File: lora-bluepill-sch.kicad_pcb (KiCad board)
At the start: 2 copper layers, 100 x 80 mm, 63 parts, among them J1 Conn_01x05, J10 Screw_Terminal_01x04, J11 Screw_Terminal_01x04, J2 Conn_01x05, J4 Conn_01x04_Male, J5 Conn_01x02, J7 Screw_Terminal_01x02, J8 Screw_Terminal_01x02, Q1 BC558, U10 YAAJ_WeAct_BlackPill_Part_Like, U2 FTDI_Breakout, U3 RadioEnge_LoRaWAN, U4 PC817, U5 PC817, U6 PC817, U7 PC817, U8 PC817, U9 NE555P

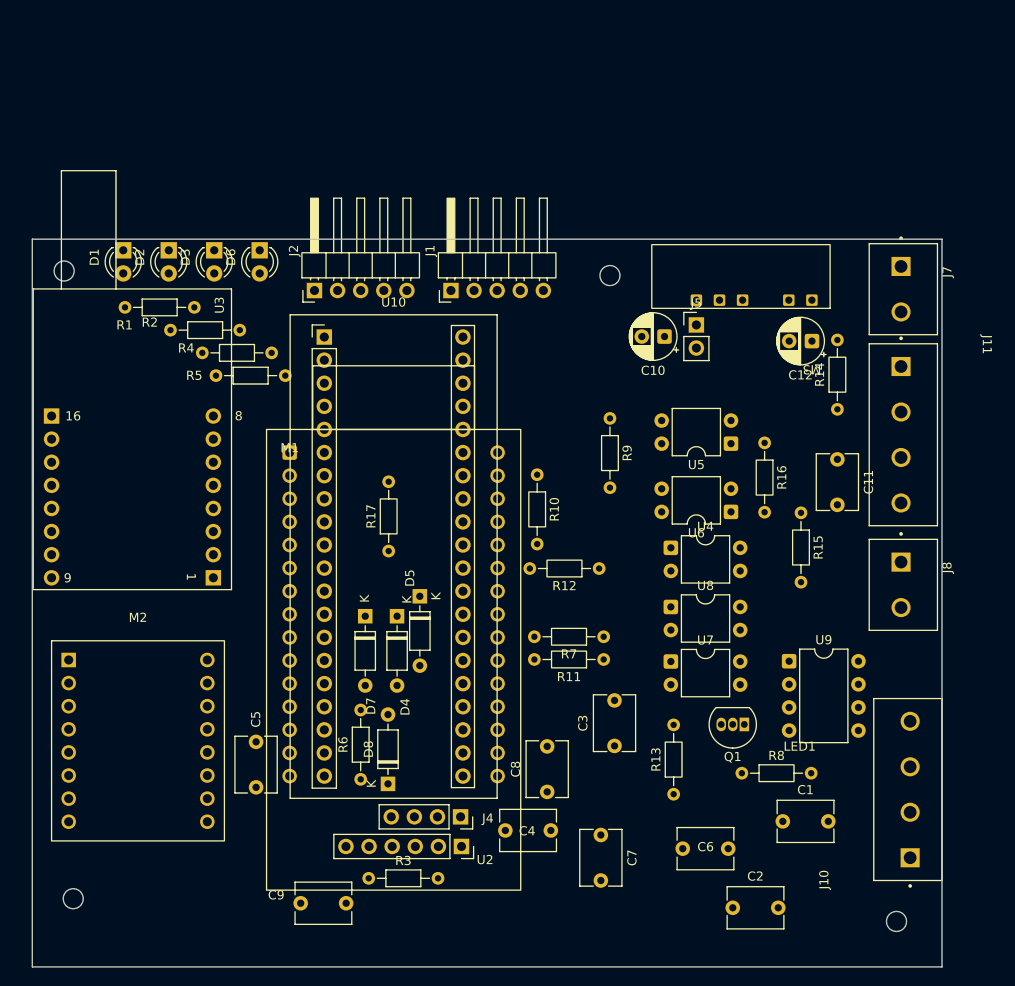
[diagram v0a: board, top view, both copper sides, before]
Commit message: board finished, but not checked
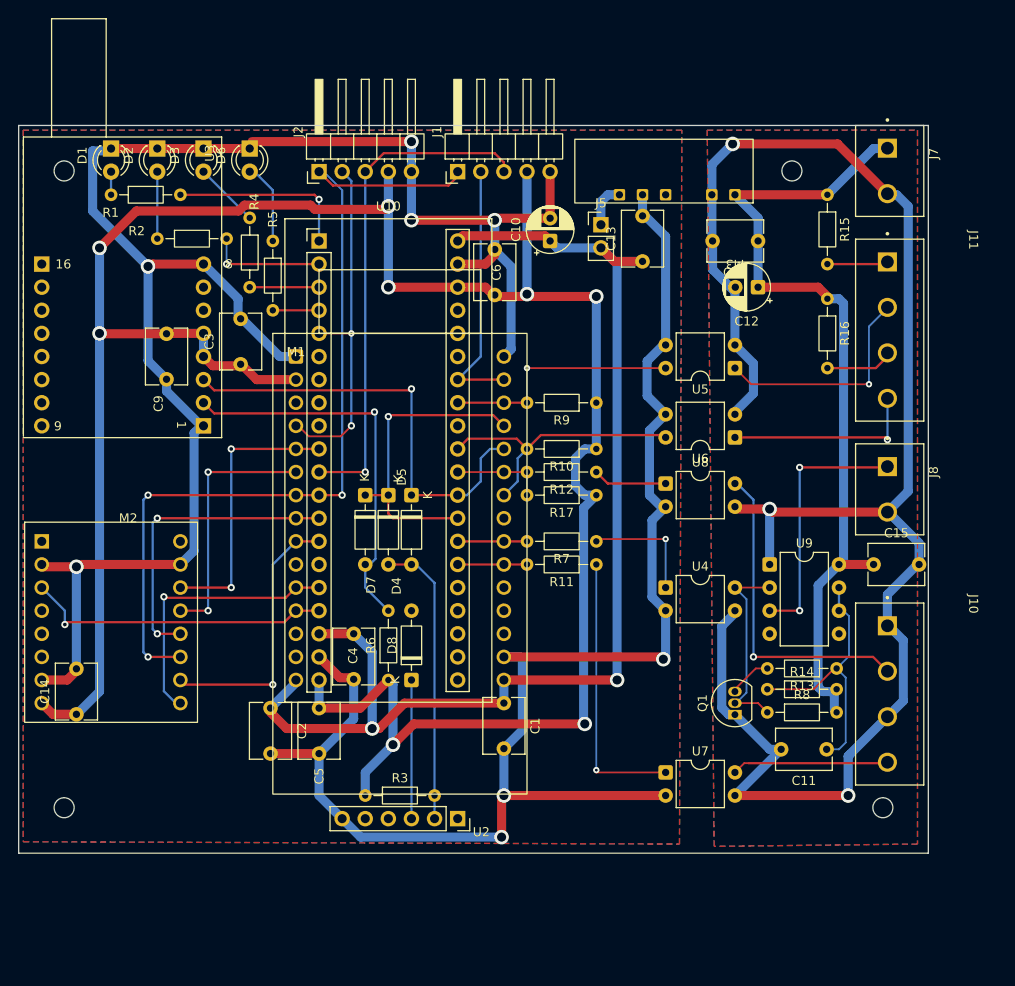
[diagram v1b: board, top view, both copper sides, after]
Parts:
- removed C7, C8: 100n, Capacitor_THT:C_Disc_D6.0mm_W4.4mm_P5.00mm
- removed J4: Conn_01x04_Male, Connector_PinSocket_2.54mm:PinSocket_1x04_P2.54mm_Vertical
- added C13: 100n, Capacitor_THT:C_Disc_D6.0mm_W4.4mm_P5.00mm, F.Cu at (68.6, 14.9)
- added C14: 100n, Capacitor_THT:C_Disc_D6.0mm_W4.4mm_P5.00mm, F.Cu at (6.35, 64.7)
- added C15: 100n, Capacitor_THT:C_Disc_D6.0mm_W4.4mm_P5.00mm, F.Cu at (94.0, 48.3)
- added C16: 100n, Capacitor_THT:C_Disc_D6.0mm_W4.4mm_P5.00mm, F.Cu at (81.3, 12.7)
- moved C6 66.1 mm to (52.3, 18.6), turned to 90 degrees
- moved C9 65.6 mm to (16.3, 22.9), turned to -90 degrees
- moved C3 58.7 mm to (24.4, 26.3)
- moved C2 55.4 mm to (27.7, 64.0), turned to -90 degrees
- moved R15 35.1 mm to (88.9, 7.62)
- moved C1 33.3 mm to (53.3, 63.5), turned to -90 degrees
- moved C11 31.9 mm to (88.8, 68.6), turned to 180 degrees
- moved R14 31.7 mm to (82.3, 62.0), turned to 0 degrees
- moved C4 27.3 mm to (36.8, 55.9), turned to -90 degrees
- moved J10 25.6 mm to (95.5, 55.0), turned to -90 degrees
- moved R17 23.6 mm to (63.5, 40.6), turned to 180 degrees
- moved H3 23.1 mm to (85.0, 5.00)
- moved R13 22.6 mm to (89.9, 59.7), turned to 180 degrees
- moved R16 17.3 mm to (88.9, 19.1)
- moved U3 16.7 mm to (20.3, 33.0)
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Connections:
- net /FTDI_RX renamed Net-(D4-A)
- J10 pad 1: /OUT1_OC -> HI_GND
- J10 pad 2: HI_GND -> /OUT2_OC
- J10 pad 3: /OUT2_OC -> HI_GND
- J10 pad 4: HI_GND -> /OUT1_OC
- M1 pad 18: unconnected-(M1-D9-Pad18) -> /EXP_C6_TX
- M1 pad 19: unconnected-(M1-D18-Pad19) -> /EXP_C6_SCL
- M1 pad 20: unconnected-(M1-D19-Pad20) -> /EXP_C6_SDA
- M1 pad 23: /UART_AT_TX -> /EXP_C6_RX
- M1 pad 24: /UART_AT_RX -> /IN2_3V3
- M1 pad 26: /IN2_3V3 -> /UART_AT_RX
- M1 pad 27: unconnected-(M1-TX-Pad27) -> /UART_AT_TX
- U10 pad 5: unconnected-(U10-PA8-Pad5) -> /TEMP1_SSEL
- U10 pad 9: /TEMP1_SSEL -> unconnected-(U10-PA12-Pad9)
- U2 pad 4: /FTDI_5V -> unconnected-(U2-VCC-Pad4)
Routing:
- net GND: track 0.00 -> 348.4 mm, vias 0 -> 8
- net +3V3: track 0.00 -> 262.5 mm, vias 0 -> 8
- net HI_GND: track 0.00 -> 189.2 mm, vias 0 -> 3
- net +5V: track 0.00 -> 131.2 mm, vias 0 -> 2
- net /MISO: track 0.00 -> 97.0 mm, vias 0 -> 3
- net +12V: track 0.00 -> 90.6 mm
- net /SCLK: track 0.00 -> 83.1 mm, vias 0 -> 3
- net /UART_AT_RX: track 0.00 -> 49.9 mm, vias 0 -> 1
- net Net-(D7-A): track 0.00 -> 42.7 mm, vias 0 -> 1
- net /TEMP1_SSEL: track 0.00 -> 38.0 mm, vias 0 -> 2
- net /OUT2_OC: track 0.00 -> 34.8 mm, vias 0 -> 1
- net /UART_AT_TX: track 0.00 -> 34.5 mm, vias 0 -> 1
- net /LR1121_IRQ: track 0.00 -> 33.7 mm, vias 0 -> 1
- net /MOSI: track 0.00 -> 33.4 mm, vias 0 -> 2
- net Net-(D4-A): track 0.00 -> 31.8 mm
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- added copper zone on B.Cu, net GND
- added copper zone on F.Cu, net GND
- added copper zone on B.Cu, net HI_GND
- added copper zone on F.Cu, net HI_GND
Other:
- board text removed: "LED1"
